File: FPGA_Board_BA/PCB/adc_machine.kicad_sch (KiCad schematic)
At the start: 21 parts, among them J19 PinHeader_03_male, Q6 NTR5103NT1G, U15 LTC2320-16_CMOS

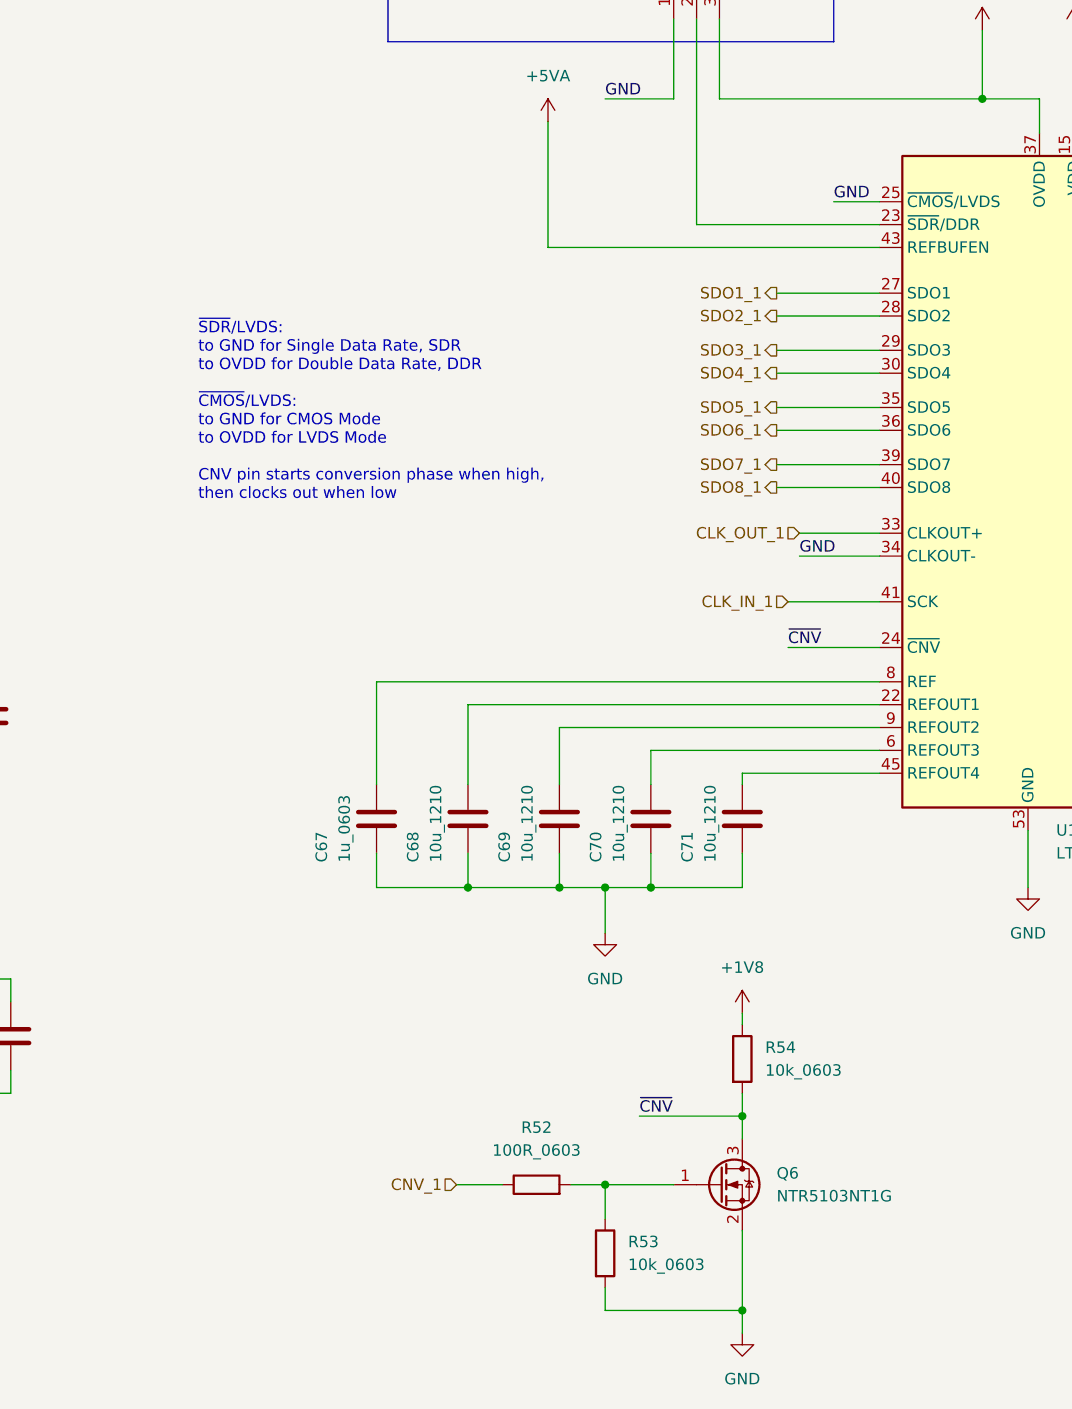
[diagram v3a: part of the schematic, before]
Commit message: 18.11 Bib Session
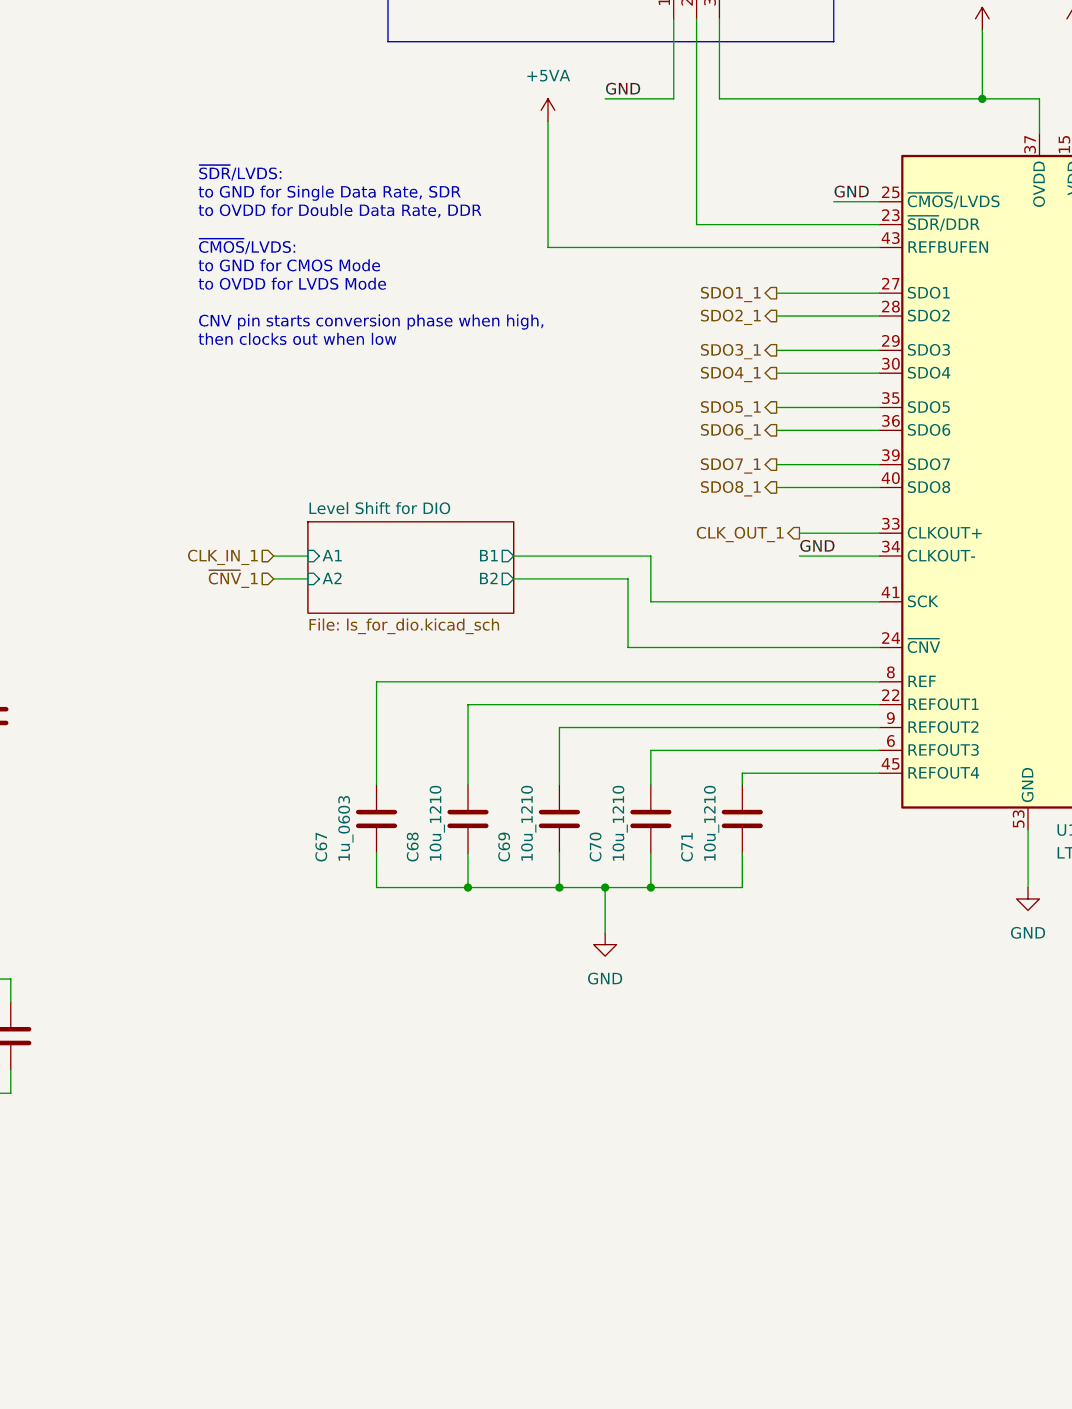
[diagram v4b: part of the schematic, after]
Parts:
- removed Q6: NTR5103NT1G, Package_TO_SOT_SMD:SOT-23_Handsoldering, symbol WLIB_Q:NTR5103NT1G
- removed R52: 100R_0603, Resistor_SMD:R_0603_1608Metric, symbol WLIB_R:100R_0603
- removed R53, R54: 10k_0603, Resistor_SMD:R_0603_1608Metric, symbol WLIB_R:10k_0603
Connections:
- net CLK_IN_1: no longer U15.41 (SCK)
- net ~{CNV} renamed Level Shift for DIO/B2
- new net Level Shift for DIO/B1: U15.41 (SCK)
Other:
- added sheet Level Shift for DIO (ls_for_dio.kicad_sch)
